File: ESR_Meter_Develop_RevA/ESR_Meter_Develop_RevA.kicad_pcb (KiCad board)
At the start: 2 copper layers, 50 x 40 mm, 23 parts, among them U1 TL074HIDR

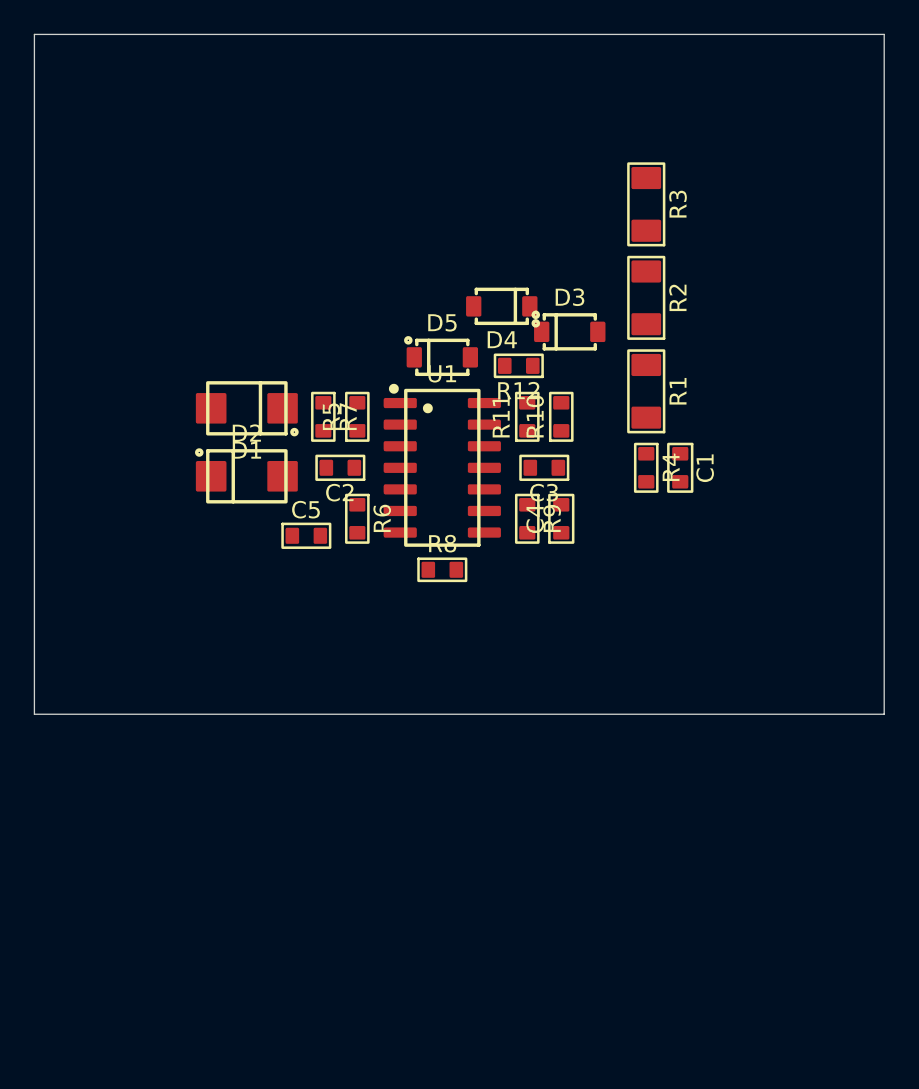
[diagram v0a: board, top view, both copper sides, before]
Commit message: working on frontend
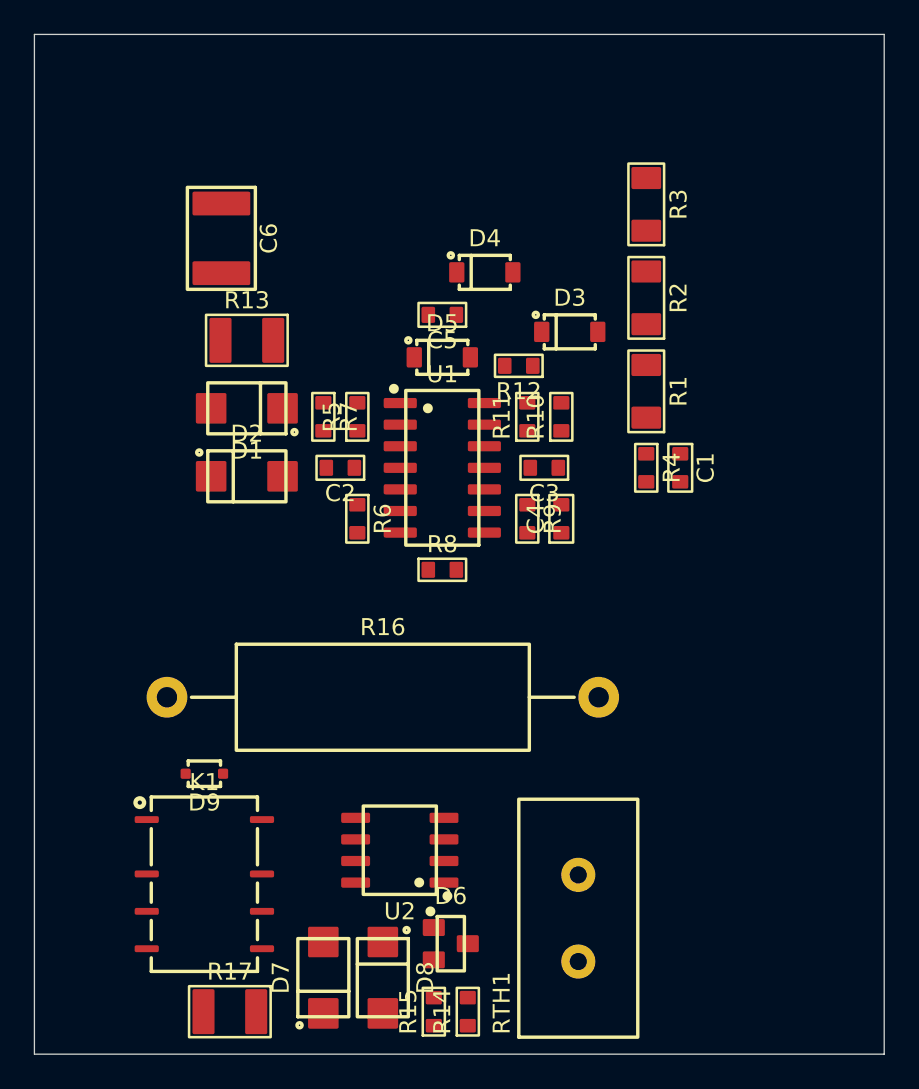
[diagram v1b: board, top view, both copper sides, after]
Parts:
- added C6: 22nF 2kV, 3Brain_Capacitors:C_1812, F.Cu at (91.0, 77.0)
- added D6: BAV99, 3Brain_Diodes:SOT-23_ACAC, F.Cu at (104.5, 118.5)
- added D7: M1, 3Brain_Diodes:D_SMA, F.Cu at (97.0, 120.5)
- added D8: M1, 3Brain_Diodes:D_SMA, F.Cu at (100.5, 120.5)
- added D9: SD12C-01FTG, 3Brain_Diodes:D_SOD-323_Bipolar, F.Cu at (90.0, 108.5)
- added K1: 1462038-4, 3Brain_Miscellaneous:AXICOM_Relay_IM, F.Cu at (90.0, 115.0)
- added R13: 2.2k, 3Brain_Resistors:R_1210, F.Cu at (92.5, 83.0)
- added R14: 1k, 3Brain_Resistors:R_0603, F.Cu at (105.5, 122.5)
- added R15: 220R, 3Brain_Resistors:R_0603, F.Cu at (103.5, 122.5)
- added R16: 1k, 3Brain_Resistors:R_Axial__L17.0mm_D6.0mm_P25.40mm_H, F.Cu at (100.5, 104.0)
- added R17: 100R, 3Brain_Resistors:R_1210, F.Cu at (91.5, 122.5)
- added RTH1: 1k, 3Brain_Miscellaneous:PTCEL13, F.Cu at (112.0, 117.0)
- added U2: TL071H, 3Brain_ICs:SOIC-8, F.Cu at (101.5, 113.0)
- moved C5 15.3 mm to (104.0, 81.5), turned to 180 degrees
- moved D4 2.24 mm to (106.5, 79.0), turned to 0 degrees
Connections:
- net Net-(U1E-V+) renamed VDD
- net Net-(U1E-V-) renamed VSS
- R3 pad 1: unconnected-(R3-Pad1) -> Net-(C6-Pad1)
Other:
- board size 50 x 40 mm -> 50 x 60 mm

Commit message: bckp
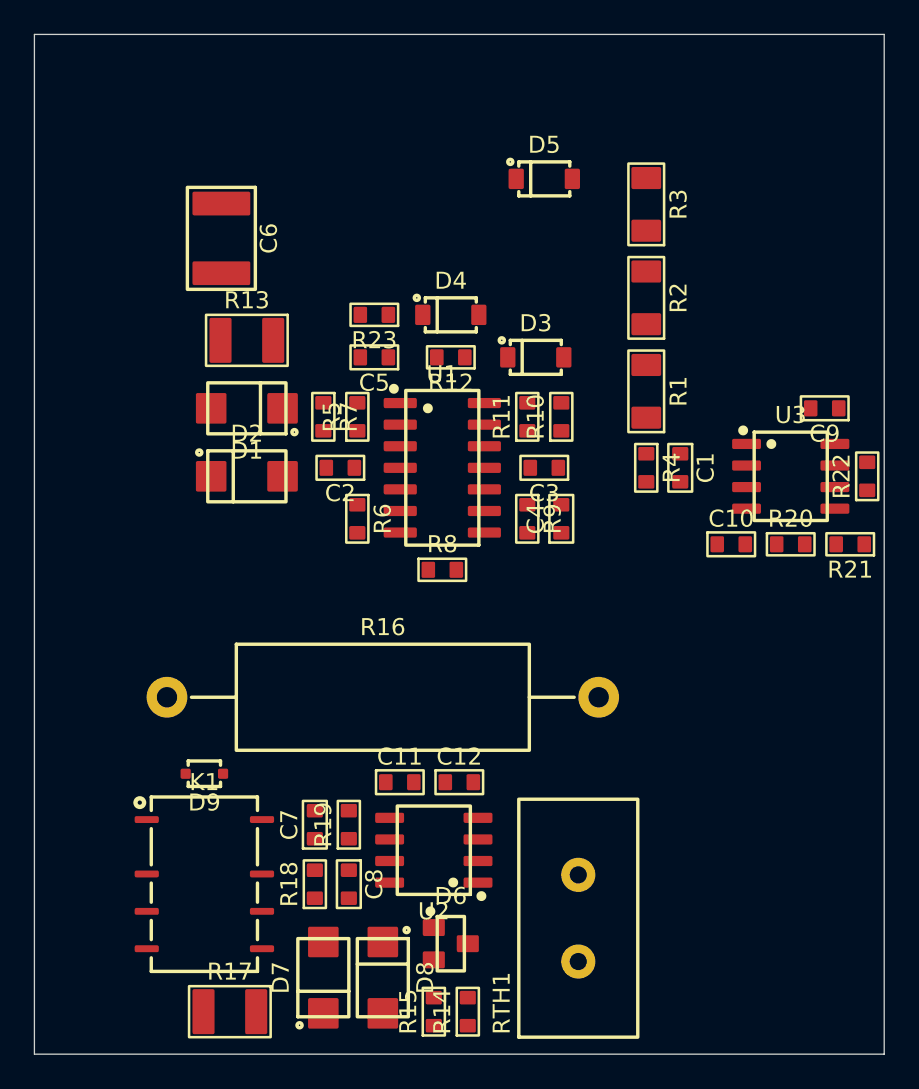
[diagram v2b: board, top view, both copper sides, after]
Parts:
- added C10: 100nF, 3Brain_Capacitors:C_0603, F.Cu at (121.0, 95.0)
- added C11: 100nF, 3Brain_Capacitors:C_0603, F.Cu at (101.5, 109.0)
- added C12: 100nF, 3Brain_Capacitors:C_0603, F.Cu at (105.0, 109.0)
- added C7: 100pF, 3Brain_Capacitors:C_0603, F.Cu at (96.5, 111.5)
- added C8: 1uF, 3Brain_Capacitors:C_0603, F.Cu at (98.5, 115.0)
- added C9: 100nF, 3Brain_Capacitors:C_0603, F.Cu at (126.5, 87.0)
- added R18: 18k, 3Brain_Resistors:R_0603, F.Cu at (96.5, 115.0)
- added R19: 2k, 3Brain_Resistors:R_0603, F.Cu at (98.5, 111.5)
- added R20: 10k, 3Brain_Resistors:R_0603, F.Cu at (124.5, 95.0)
- added R21: 10k, 3Brain_Resistors:R_0603, F.Cu at (128.0, 95.0)
- added R22: 10k, 3Brain_Resistors:R_0603, F.Cu at (129.0, 91.0)
- added R23: 10k, 3Brain_Resistors:R_0603, F.Cu at (100.0, 81.5)
- added U3: TL072H, 3Brain_ICs:SOIC-8, F.Cu at (124.5, 91.0)
- moved D5 12.1 mm to (110.0, 73.5)
- moved C5 4.72 mm to (100.0, 84.0)
- moved R12 4.03 mm to (104.5, 84.0)
- moved D4 3.20 mm to (104.5, 81.5)
- moved D3 2.50 mm to (109.5, 84.0)
- moved U2 2.00 mm to (103.5, 113.0)
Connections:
- U2 pad 3: unconnected-(U2-+-Pad3) -> Net-(U2-+)
